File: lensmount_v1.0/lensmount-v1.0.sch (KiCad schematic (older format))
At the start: 43 parts, among them J1 VBAT, J10 Picoblade DNP, J2 DETECT, J3 AGND, J4 VDD, J5 DOUT, J6 DIN, J7 DCLK, J8 DGND, J9 USB, P1 TC2030-CTX-Tag-Connect, Q1 2N7002, Q2 2N7002, Q3 2N7002, Q4 AO3401A, Q5 AO3401A, U1 STM32F042F6Px, U2 XC6206PxxxMR, U3 USBLC6-4

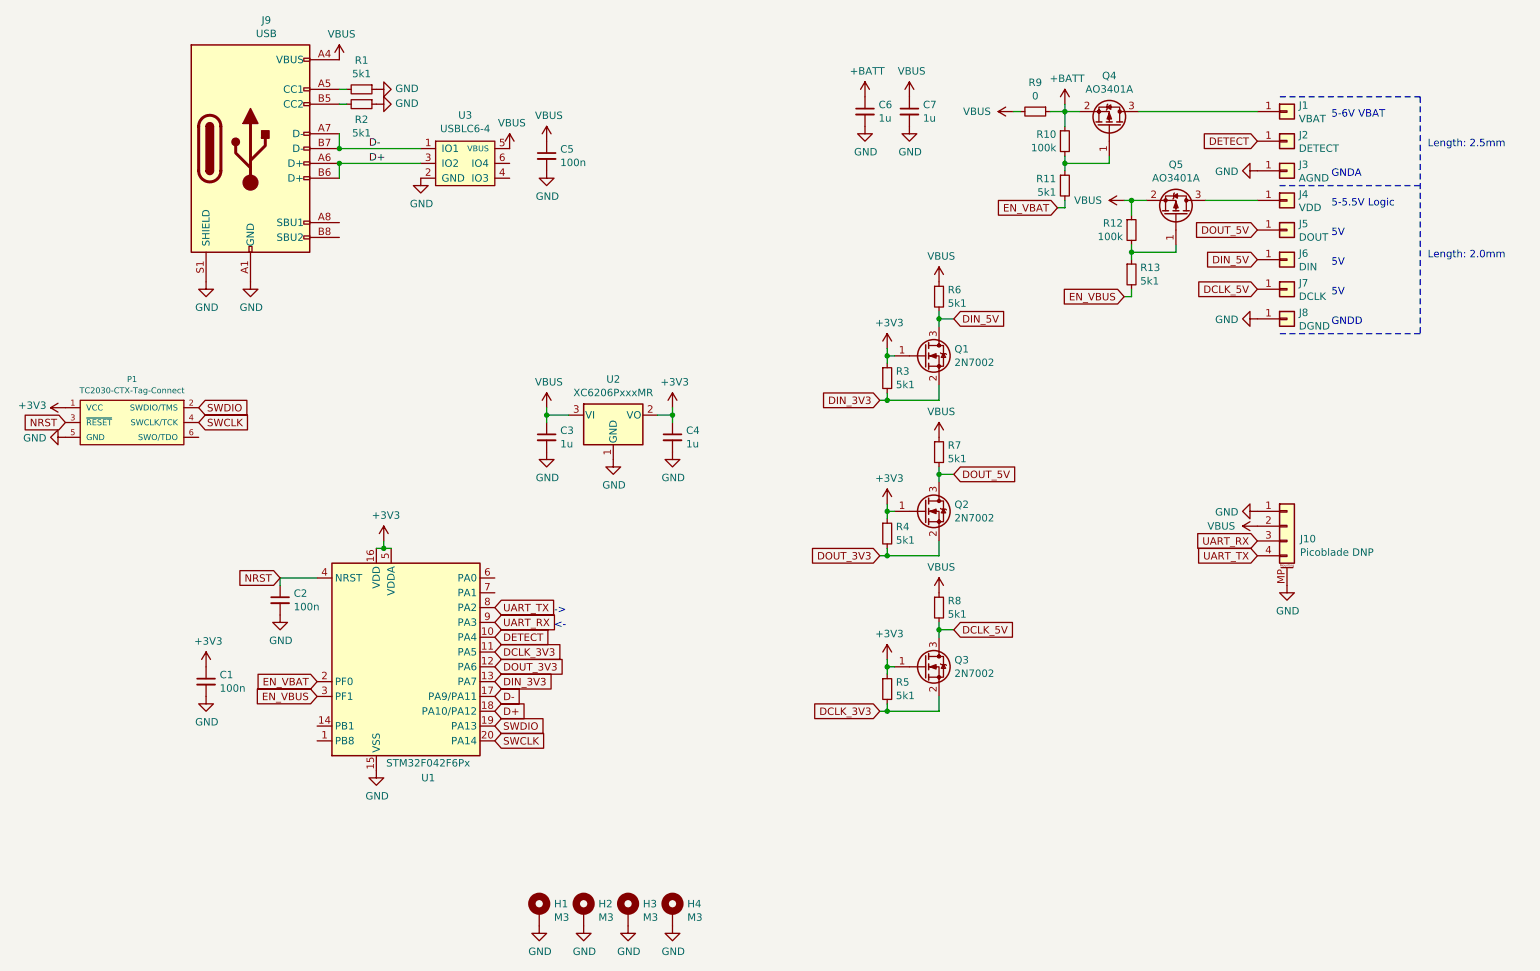
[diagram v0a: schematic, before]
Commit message: added all gerber
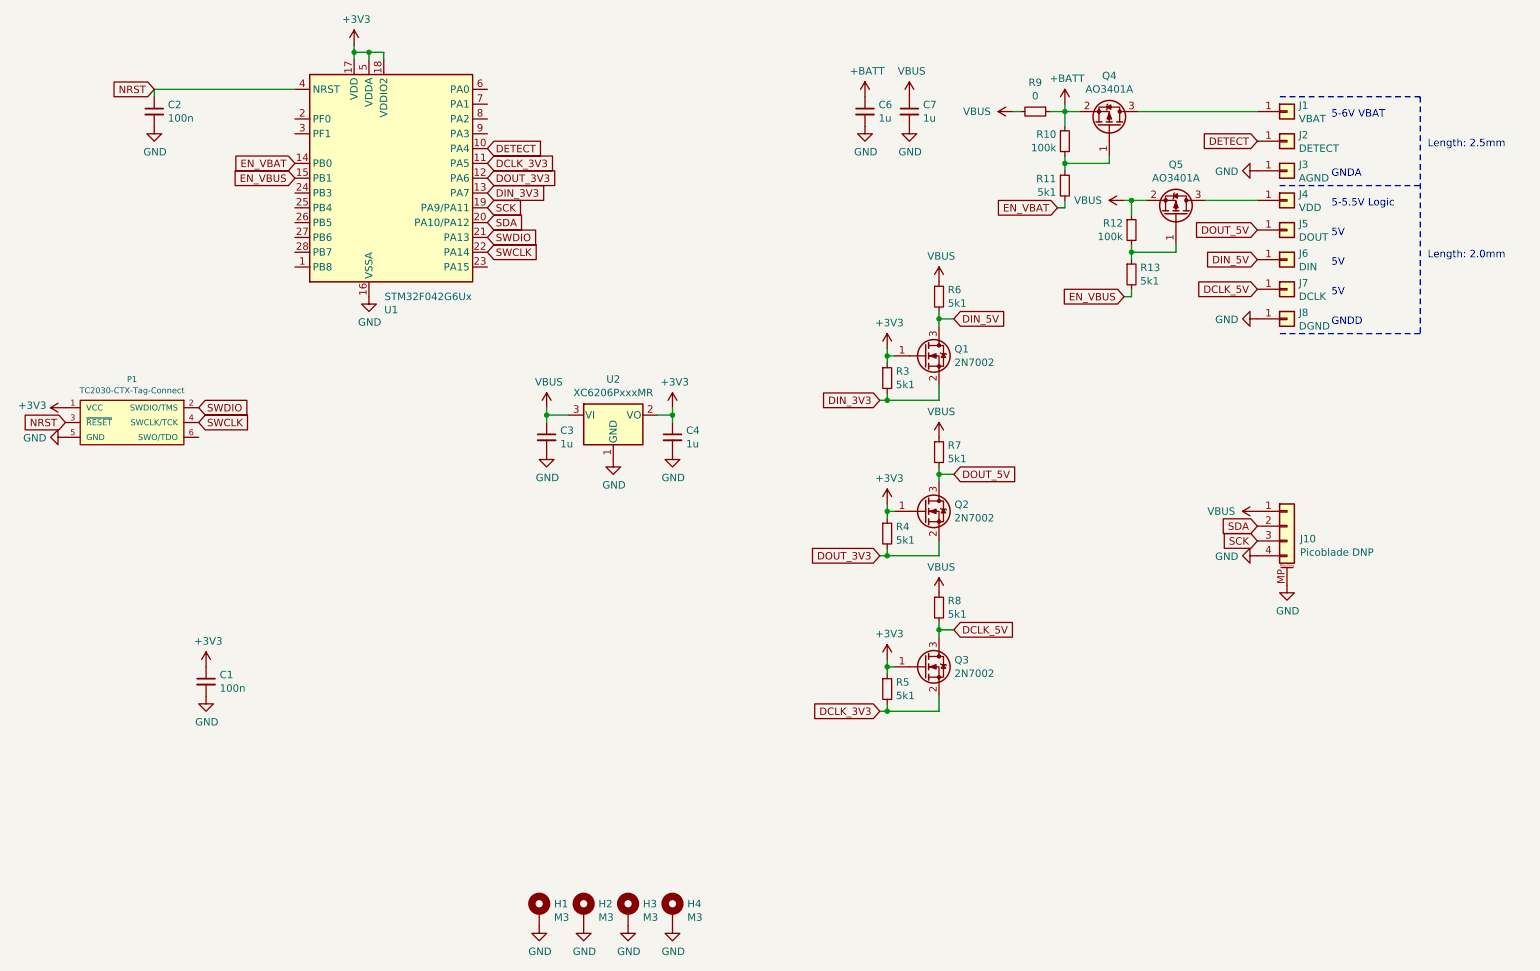
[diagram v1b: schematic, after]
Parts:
- removed C5: 100n, otter:C_0402, symbol Device:C_Small
- removed J9: USB, otter:USB-C 16Pin, symbol Connector:USB_C_Receptacle_USB2.0
- removed R1, R2: 5k1, otter:R_0402, symbol Device:R_Small
- removed U1: STM32F042F6Px, Package_SO:TSSOP-20_4.4x6.5mm_P0.65mm, symbol MCU_ST_STM32F0:STM32F042F6Px
- removed U3: USBLC6-4, Package_TO_SOT_SMD:SOT-23-6, symbol otter:otter_USBLC6-4
- added U1: STM32F042G6Ux, Package_DFN_QFN:QFN-28_4x4mm_P0.5mm, symbol MCU_ST_STM32F0:STM32F042G6Ux
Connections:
- net UART_TX is gone; now on net GND: J10.4 (Pin_4)
- net +3V3: now also U1.17 (VDD), U1.18 (VDDIO2), U1.5 (VDDA)
- net DCLK_3V3: now also U1.11 (PA5)
- net DETECT: now also U1.10 (PA4)
- net DIN_3V3: now also U1.13 (PA7)
- net DOUT_3V3: now also U1.12 (PA6)
- net EN_VBAT: now also U1.14 (PB0)
- net EN_VBUS: now also U1.15 (PB1)
- net GND: now also U1.16 (VSSA); no longer J10.1 (Pin_1)
- net NRST: now also U1.4 (NRST)
- net SWCLK: now also U1.22 (PA14)
- net SWDIO: now also U1.21 (PA13)
- net VBUS: now also J10.1 (Pin_1); no longer J10.2 (Pin_2)
- net UART_RX renamed SCK
- net SCK: now also U1.19 (PA9/PA11)
- new net SDA: J10.2 (Pin_2), U1.20 (PA10/PA12)
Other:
- note removed: "->"
- note removed: "<-"
- moved on the sheet: C2
